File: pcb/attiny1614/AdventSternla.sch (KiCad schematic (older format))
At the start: 15 parts, among them J1 5V In, J2 GPIO_C, J3 UPDI, J4 GPIO_A, J5 NeoPixel, J6 GPIO_A, J7 GPIO_B, U1 ATTINY1614

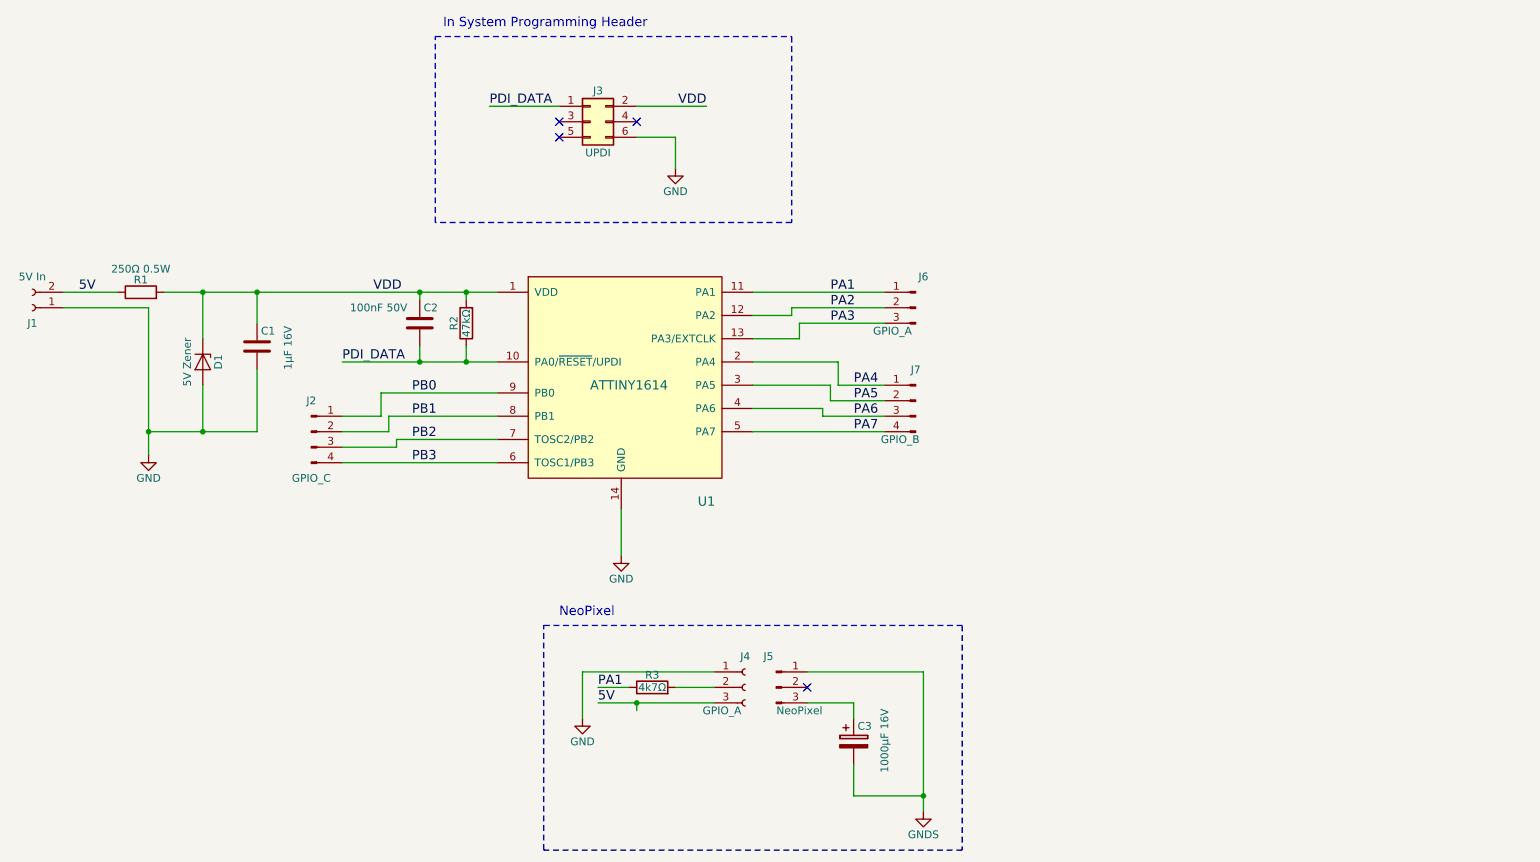
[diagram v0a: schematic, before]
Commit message: Schematic is done and started the layout
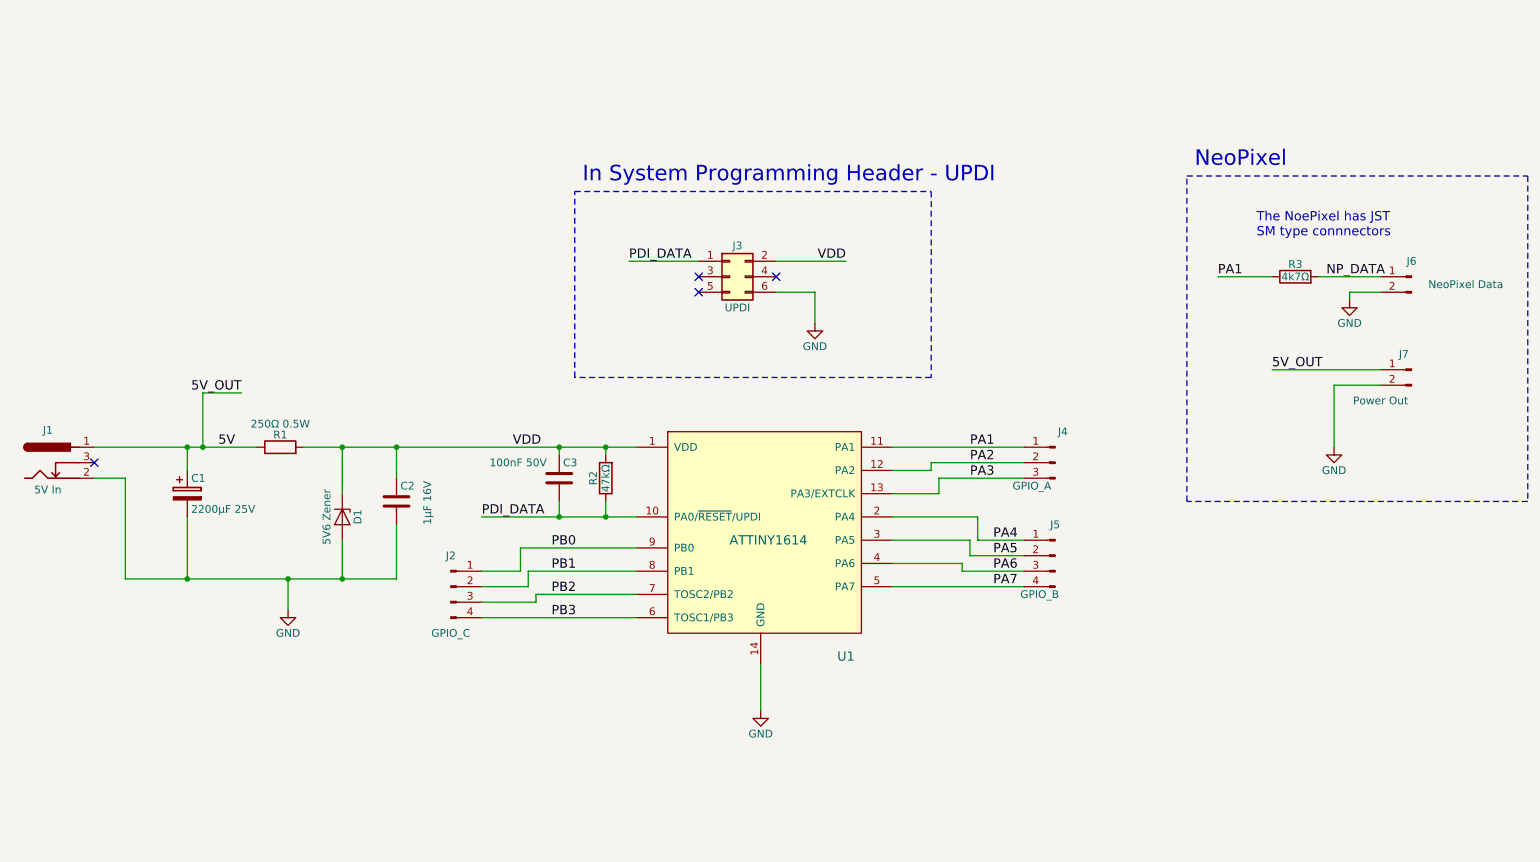
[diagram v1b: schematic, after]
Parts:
- removed C3: 1000μF 16V, symbol CP
- removed J1: 5V In, symbol Conn_01x02_Female
- removed J4: GPIO_A, symbol Conn_01x03_Female
- removed J5: NeoPixel, symbol Conn_01x03_Male
- added C1: 2200μF 25V, Capacitors_ThroughHole:CP_Radial_D13.0mm_P5.00mm, symbol CP
- added J1: 5V In, Pin_Headers:Pin_Header_Straight_1x03_Pitch2.54mm, symbol Jack-DC
- added J6: NeoPixel Data, Pin_Headers:Pin_Header_Straight_1x02_Pitch2.54mm, symbol Conn_01x02_Male
- added J7: Power Out, Pin_Headers:Pin_Header_Straight_1x02_Pitch2.54mm, symbol Conn_01x02_Male
- C2: renamed from C1; footprint 0805 -> Capacitors_SMD:C_0805_HandSoldering
- C3: renamed from C2; footprint (none) -> Capacitors_SMD:C_0805_HandSoldering
- D1: value 5V Zener -> 5V6 Zener; footprint DO-214AA -> Diodes_SMD:D_SOT-23_ANK; Link https://www.reichelt.de/Ueberspannungs-schutzdioden/P6SMB-5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 -> https://www.digikey.de/scripts/DkSearch/dksus.dll?Detail&it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; MPN P6SMB 5,0A SMD -> BZX84-A5V6,215
- J2: footprint (none) -> Pin_Headers:Pin_Header_Straight_1x04_Pitch2.54mm
- J3: footprint (none) -> Pin_Headers:Pin_Header_Straight_2x03_Pitch2.54mm
- J4: renamed from J6; footprint (none) -> Pin_Headers:Pin_Header_Straight_1x03_Pitch2.54mm
- J5: renamed from J7; footprint (none) -> Pin_Headers:Pin_Header_Straight_1x04_Pitch2.54mm
- R1: footprint 1210 -> Resistors_SMD:R_1210_HandSoldering
- R2: footprint 0805 -> Resistors_SMD:R_0805_HandSoldering
- R3: footprint (none) -> Resistors_SMD:R_0805_HandSoldering
- U1: footprint (none) -> SMD_Packages:SOIC-14_N
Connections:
- net 5V: now also C1.1, J1.1, J7.1 (Pin_1)
- net GND: now also C1.2, J1.2, J6.2 (Pin_2), J7.2 (Pin_2)
- net NP_DATA: now reaches R3.2
- net NP_DATA: now also J6.1 (Pin_1)
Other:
- note added: "In System Programming Header - UPDI"
- note added: "The NoePixel has JST \nSM type connnectors"
- note removed: "In System Programming Header"
- moved on the sheet: C2, C3, D1, J2, J3, J4, J5, R1, R2, R3, U1
